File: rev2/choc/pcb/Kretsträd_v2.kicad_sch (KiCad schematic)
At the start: 49 parts, among them J1 Conn_01x02_Female, J2 Conn_01x02_Female, J3 Conn_01x01_Socket, J4 Conn_01x01_Socket, SW1 ${REFERENCE}, SW10 ${REFERENCE}, SW11 ${REFERENCE}, SW12 ${REFERENCE}, SW13 ${REFERENCE}, SW14 ${REFERENCE}, SW15 ${REFERENCE}, SW16 ${REFERENCE}, SW17 ${REFERENCE}, SW2 ${REFERENCE}, SW3 ${REFERENCE}, SW4 ${REFERENCE}, SW5 ${REFERENCE}, SW6 ${REFERENCE}, SW7 ${REFERENCE}, SW8 ${REFERENCE}, SW9 ${REFERENCE}, U1 SeeeduinoXIAO_nRF52840

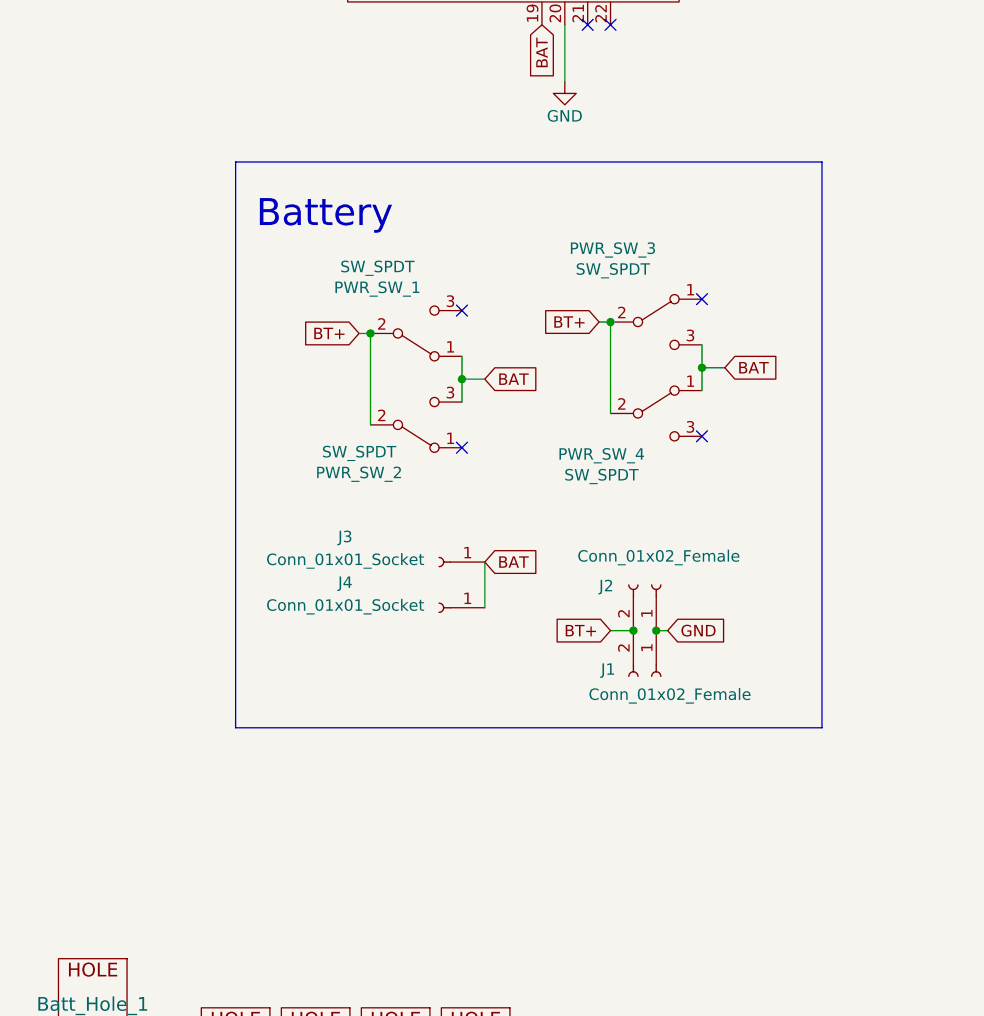
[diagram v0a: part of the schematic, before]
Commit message: v2.2
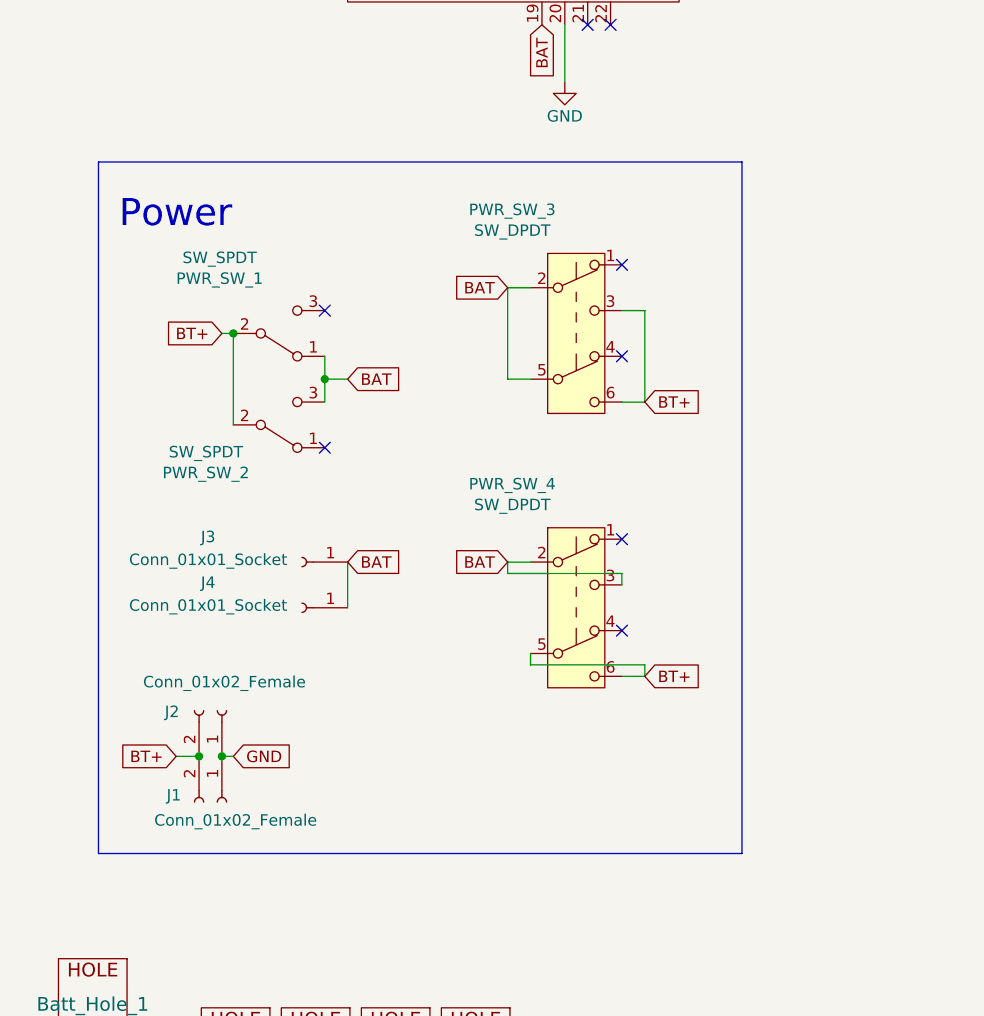
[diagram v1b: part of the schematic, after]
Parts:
- removed PWR_SW_4: SW_SPDT, Button_Switch_SMD:SW_SPDT_PCM12, symbol Switch:SW_SPDT
- added PWR_SW_4: SW_DPDT, jw_custom_footprints:Button_Switch_Push_Horizontal_2P2T_Toggle_5.8x5.8, symbol Switch:SW_Push_DPDT
- D1, D10, D11, D12, D13, D14, D15, D16, D17, D2, D3, D4, D5, D6, D7, D8, D9: footprint jw_custom_footprints:Diode_SOD123_THT_2 -> jw_custom_footprints:Diode_SOD123_THT_v3
- PWR_SW_3: value SW_SPDT -> SW_DPDT; footprint Button_Switch_SMD:SW_SPDT_PCM12 -> jw_custom_footprints:Button_Switch_Push_Vertical_2P2T_Toggle_5.8x5.8; symbol Switch:SW_SPDT -> Switch:SW_Push_DPDT
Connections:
- net BAT: now also PWR_SW_3.2 (B), PWR_SW_3.5 (B), PWR_SW_4.2 (B), PWR_SW_4.3 (C); no longer PWR_SW_3.3 (C)
- net BT+: now also PWR_SW_3.3 (C), PWR_SW_3.6 (C), PWR_SW_4.5 (B), PWR_SW_4.6 (C); no longer PWR_SW_3.2 (B)
- no-connect marks 12 -> 14
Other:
- note added: "Power"
- note removed: "Battery"
- moved on the sheet: J1, J2, J3, J4, PWR_SW_1, PWR_SW_2
